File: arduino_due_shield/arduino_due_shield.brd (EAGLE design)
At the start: 101.6 x 53.3 mm, 27 parts, among them J12 ARDUINO_MEGA_R3FULL, J13 POLOLU-2595, J14 POLOLU-2807, J15 POLOLU-2595

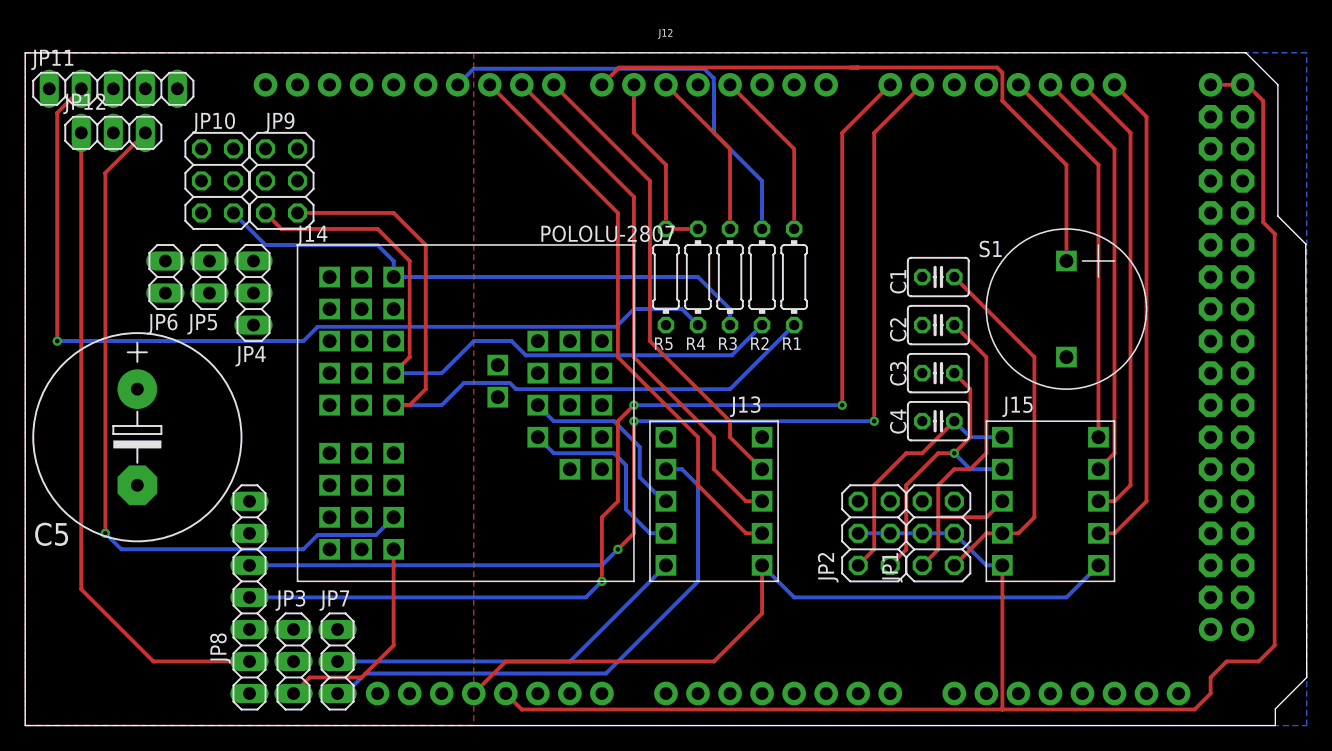
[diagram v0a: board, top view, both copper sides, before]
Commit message: Finish schematic and PCB design
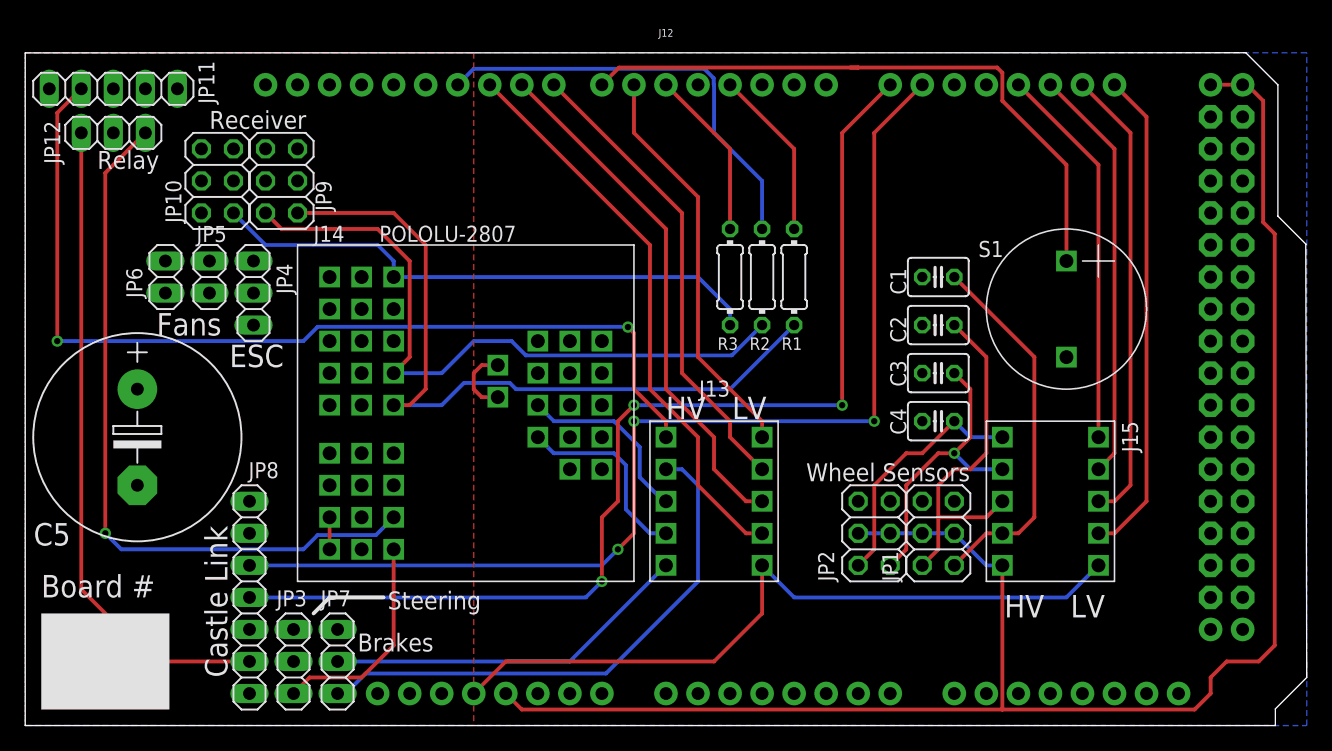
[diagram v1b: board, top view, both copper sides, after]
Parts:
- removed R4: 3.3k, resistor:0204/7
- removed R5: 2.2k, resistor:0204/7
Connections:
- net RX1 renamed RC_RX1
- net RX2 renamed RC_RX2
- net RX3 renamed RC_RX3
- removed net RELAYHV: JP11.2, R4.2
- new net N$2: J14.FAILMODE1, J14.FAILMODE2
- new net RELAYOUT_HV: J13.H4, JP11.2
- net GND: no longer R5.1
- net RELAYOUT: now also J13.L4; no longer R4.1, R5.2
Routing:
- net RELAYOUT_HV: track 0.00 -> 76.5 mm, vias 0 -> 2
- net RELAYHV: track 73.2 -> 0.00 mm, vias 1 -> 0
- net RELAYOUT: track 15.0 -> 32.1 mm
- net N$2: track 0.00 -> 5.61 mm
- net GND: track 0.00 -> 2.54 mm
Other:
- board text added: "AutoRally Arduino Due Shield, rev 1, 2019"
- board text added: "Board #"
- board text added: "Brakes"
- board text added: "Castle Link"
- board text added: "ESC"
- board text added: "Fans"
- board text added: "HV LV"
- board text added: "Receiver"
- board text added: "Relay"
- board text added: "Steering"
- board text added: "Wheel Sensors"
